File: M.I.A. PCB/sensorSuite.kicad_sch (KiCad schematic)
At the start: 13 parts, among them U3 MMC5983MA, U4 ICM-42688-P, U5 MS5611-01BA, U6 TMP117xxDRV, U7 MAX-M10S, U8 KX134-1211

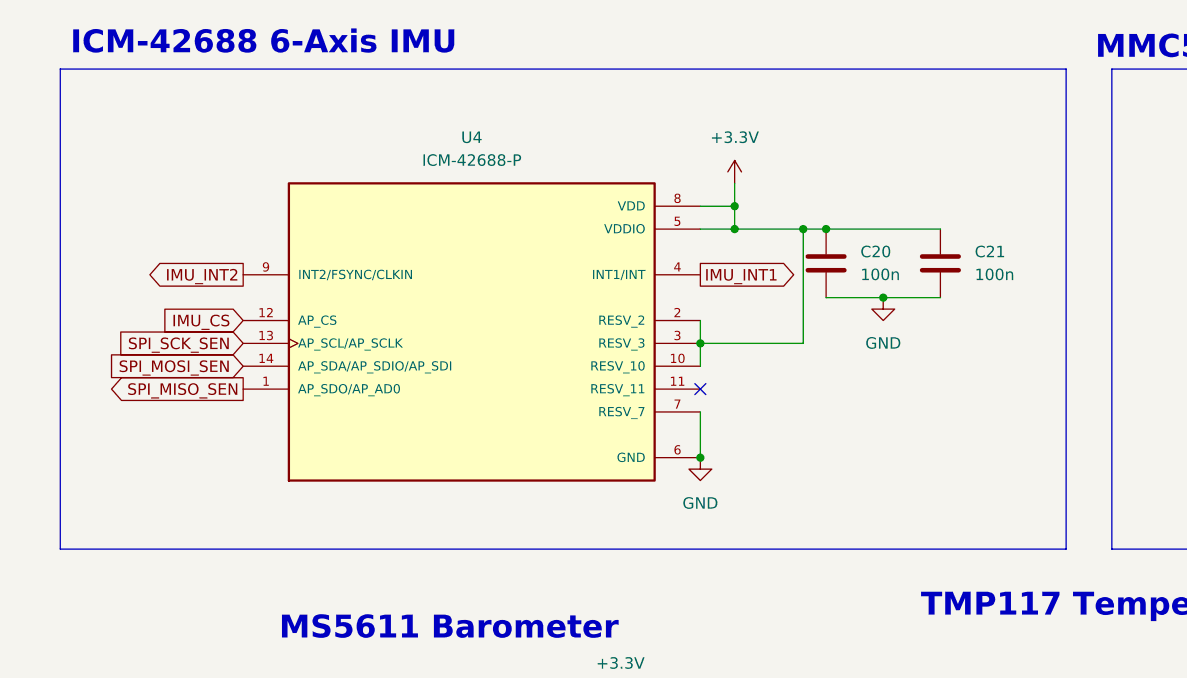
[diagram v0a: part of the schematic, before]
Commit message: Worked on Layout, Changed IMU
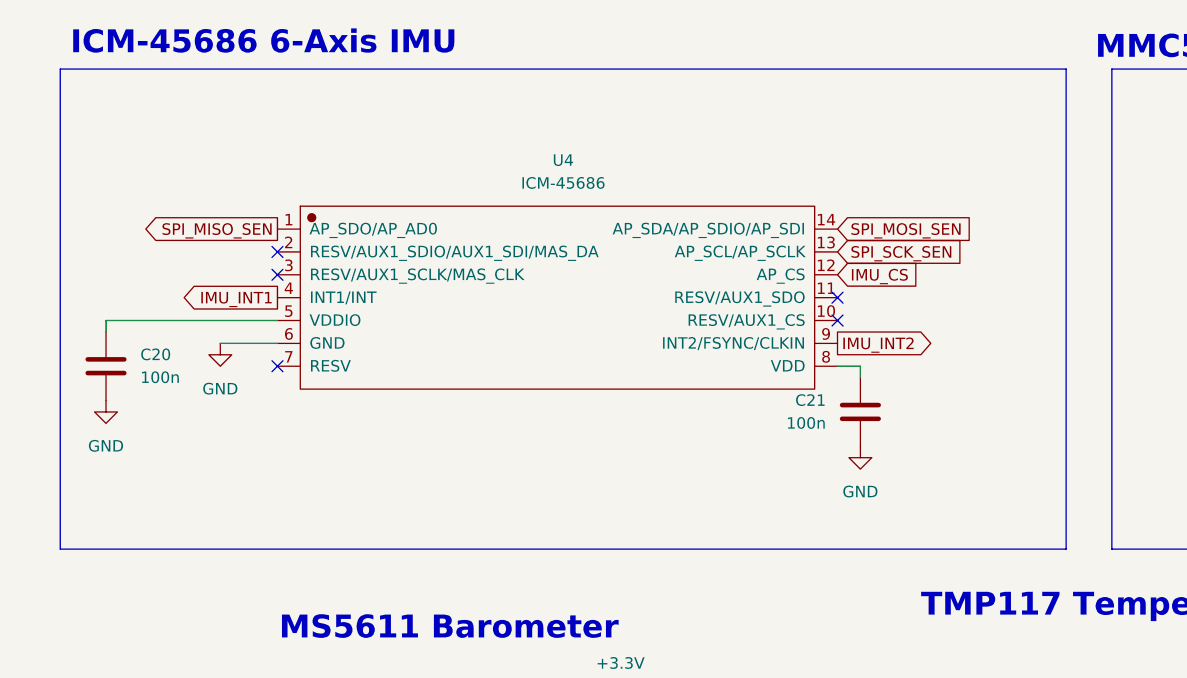
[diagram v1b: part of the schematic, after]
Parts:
- removed U4: ICM-42688-P, Package_LGA:LGA-14_3x2.5mm_P0.5mm_LayoutBorder3x4y, symbol ICM-42688-P:ICM-42688-P
- added U4: ICM-45686, Package_LGA:Bosch_LGA-14_3x2.5mm_P0.5mm, symbol JLCImport:ICM-45686
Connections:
- net +3.3V: no longer C20.1, C21.1
- net GND: now also U4.6 (GND)
- net IMU_CS: now also U4.12 (AP_CS)
- net IMU_INT1: now also U4.4 (INT1/INT)
- net IMU_INT2: now also U4.9 (INT2/FSYNC/CLKIN)
- net SPI_MISO_SEN: now also U4.1 (AP_SDO/AP_AD0)
- net SPI_MOSI_SEN: now also U4.14 (AP_SDA/AP_SDIO/AP_SDI)
- net SPI_SCK_SEN: now also U4.13 (AP_SCL/AP_SCLK)
- new net: C20.1, U4.5 (VDDIO)
- new net: C21.1, U4.8 (VDD)
- no-connect marks 2 -> 6
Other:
- note added: "ICM-45686 6-Axis IMU"
- note removed: "ICM-42688 6-Axis IMU"
